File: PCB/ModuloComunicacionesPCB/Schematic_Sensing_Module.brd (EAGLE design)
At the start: 109 x 82 mm, 72 parts, among them Q1 CSM-7X-DU, SW2 1825910-6

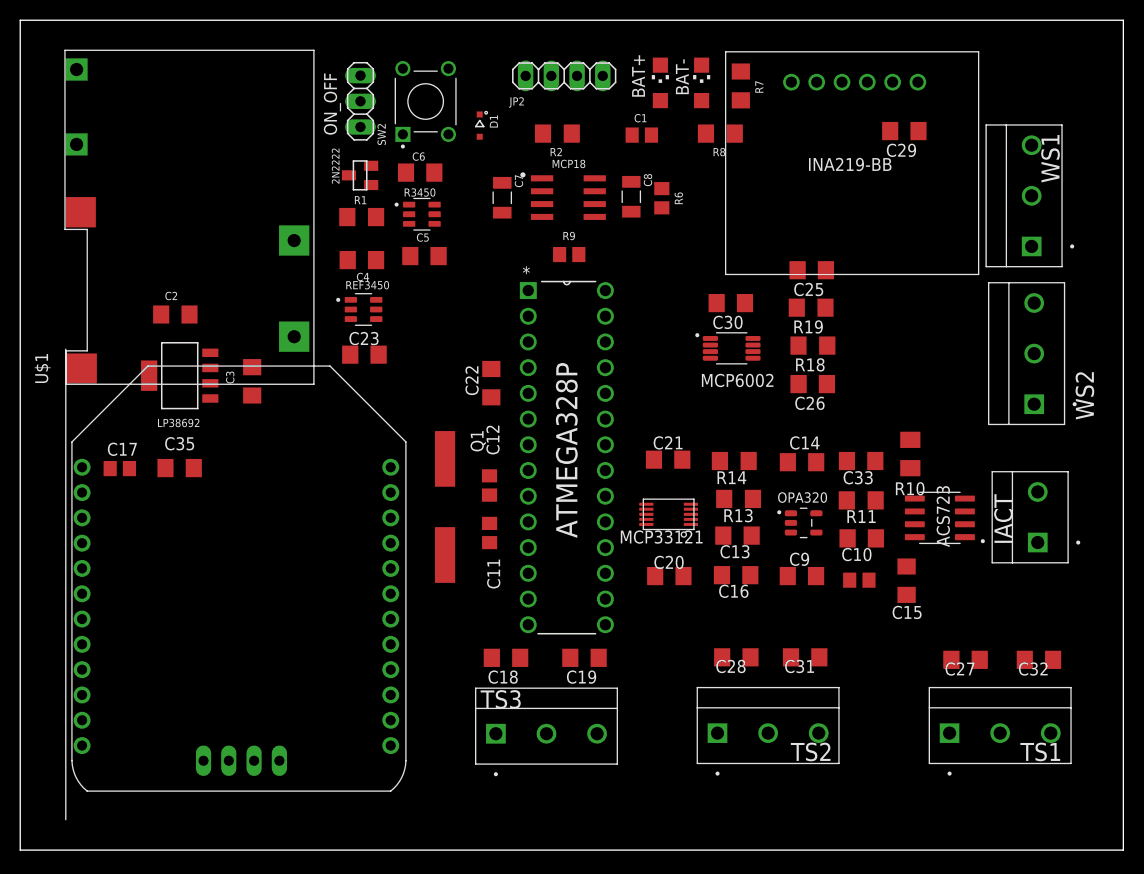
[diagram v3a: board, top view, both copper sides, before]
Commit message: pcb ruteada falta plano de tierra
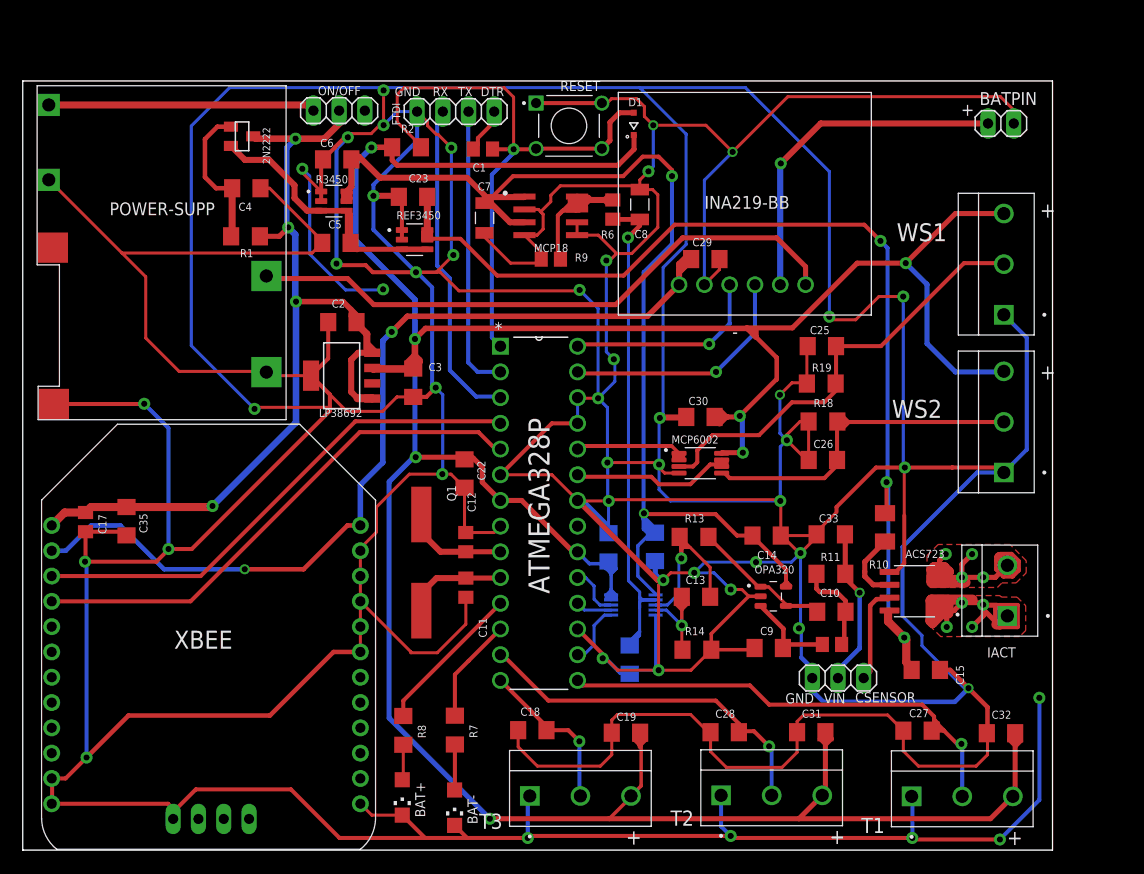
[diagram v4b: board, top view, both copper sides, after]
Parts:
- removed JP2: (no value), pinhead:1X04
- removed ON_OFF: (no value), pinhead:1X03
- removed SW2: 1825910-6, button1825910-6:SW_1825910-6-4
- removed TS1, TS2, TS3: (no value), TERMINAL-TB001:TERMINAL-TB3
- removed U$1: MODULO_CARGA_DEVICE, Modulo_Carga:MODULO_CARGA
- added BATPIN: (no value), pinhead:1X02
- added FTDI: (no value), pinhead:1X04
- added JP1, ON/OFF: (no value), pinhead:1X03
- added POWER-SUPP: MODULO_CARGA_DEVICE, Modulo_Carga:MODULO_CARGA
- added RESET: 1825910-6, button1825910-6:SW_1825910-6-4
- added T1, T2, T3: (no value), TERMINAL-TB001:TERMINAL-TB3
- moved BAT- 75.7 mm to (42.9, 4.19), turned to 180 degrees
- moved BAT+ 75.1 mm to (37.8, 5.21), turned to 180 degrees
- moved R7 69.6 mm to (43.0, 11.9)
- moved R8 66.8 mm to (37.9, 11.8), turned to 90 degrees
- moved C29 23.4 mm to (67.7, 58.4), turned to 0 degrees
- moved C21 20.1 mm to (60.2, 18.8), flipped to the bottom, turned to 90 degrees
- moved R14 19.0 mm to (66.9, 19.8)
- moved C2 16.5 mm to (31.8, 52.2)
- moved C23 16.3 mm to (38.8, 64.5)
- moved LP38692 16.0 mm to (31.8, 46.9)
- moved C3 15.9 mm to (38.8, 46.2), turned to 270 degrees
- moved C1 15.8 mm to (45.7, 69.3)
- moved D1 15.2 mm to (60.6, 71.8), turned to 90 degrees
- moved R2 15.0 mm to (38.2, 69.5), turned to 180 degrees
- moved C4 13.4 mm to (22.3, 65.4), turned to 0 degrees
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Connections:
- net N$2 renamed BASE
- removed net AMOSI: ATMEGA328P.17, MCP33121.9
- removed net VO: ACS723.7, C33.1, R11.2
- new net VIN: C33.1, JP1.2, R11.2
- new net VOACS: ACS723.7, JP1.1
- net B+INA: now also POWER-SUPP.BAT+; no longer U$1.BAT+
- net B-INA: now also BATPIN.1
- net DATAT1: now also ATMEGA328P.15, T1.2; no longer ATMEGA328P.14, TS1.2
- net DATAT2: now also ATMEGA328P.13, T2.2; no longer ATMEGA328P.15, TS2.2
- net DATAT3: now also ATMEGA328P.14, T3.2; no longer ATMEGA328P.13, TS3.2
- net DATAW1: now also WS1.2; no longer WS1.3
- net DATAW2: now also WS2.2; no longer WS2.3
- net DTR: now also FTDI.4; no longer JP2.4
- net GND: now also ATMEGA328P.17, BATPIN.2, FTDI.1, JP1.3, POWER-SUPP.BAT-, POWER-SUPP.IN-, POWER-SUPP.VOUT-, RESET.1, RESET.2, T1.1, T2.1, T3.1; no longer JP2.1, SW2.1, SW2.2, TS1.1, TS2.1, TS3.1, U$1.BAT-, U$1.IN-, U$1.VOUT-
- net RST: now also RESET.3, RESET.4; no longer SW2.3, SW2.4
- net RX0: now also FTDI.3; no longer JP2.3
- net TX0: now also FTDI.2; no longer JP2.2
- net VLP5: now also MCP33121.9, T1.3, T2.3, T3.3, WS1.3, WS2.3; no longer ATMEGA328P.21, TS1.3, TS2.3, TS3.3, WS1.2, WS2.2
- net VOUT+: now also ON/OFF.3, POWER-SUPP.VOUT+; no longer C17.1, C35.1, ON_OFF.3, U$1.VOUT+
- net VOW1: now also ATMEGA328P.24; no longer ATMEGA328P.23
- net VOW2: now also ATMEGA328P.23; no longer ATMEGA328P.24
- net VSUPPLY: now also C17.1, C35.1, ON/OFF.2, U$8.5V; no longer ON_OFF.2
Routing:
- net GND: track 0.00 -> 1286.8 mm, vias 0 -> 48
- net VLP5: track 0.00 -> 346.7 mm, vias 0 -> 7
- net VREF5: track 0.00 -> 121.0 mm, vias 0 -> 2
- net VACS: track 0.00 -> 104.3 mm, vias 0 -> 3
- net VSUPPLY: track 0.00 -> 96.5 mm, vias 0 -> 4
- net VDD33: track 0.00 -> 92.6 mm, vias 0 -> 2
- net RST: track 0.00 -> 60.7 mm, vias 0 -> 1
- net B+INA: track 0.00 -> 60.1 mm
- net VREF18: track 0.00 -> 55.1 mm, vias 0 -> 1
- net TX1: track 0.00 -> 52.0 mm
- net RX1: track 0.00 -> 50.8 mm
- net DATAT1: track 0.00 -> 48.5 mm, vias 0 -> 1
- net DATAW1: track 0.00 -> 44.1 mm
- net IP+: track 0.00 -> 36.9 mm, vias 0 -> 4
- net DATAW2: track 0.00 -> 36.6 mm
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- added copper zone on layer 1, net IP+
- added copper zone on layer 1, net IP-
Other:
- board size 109 x 82 mm -> 101.8 x 76 mm
- board text added: "+"
- board text added: "-"
- board text added: "CSENSOR"
- board text added: "DTR"
- board text added: "GND"
- board text added: "RX"
- board text added: "TX"
- board text added: "VIN"
- board text added: "XBEE"
- board text added: "ecotic"
